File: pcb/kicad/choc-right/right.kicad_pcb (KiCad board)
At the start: 2 copper layers, 135.9 x 90.2 mm, 61 parts, among them J1 USB_C_Receptacle_USB2.0, J2 AudioJack4, J3 Conn_01x12_Male, SW1 BOOT, SW10 SW_Push, SW12 SW_Push, SW13 SW_Push, SW14 SW_Push, SW15 SW_Push, SW17 SW_Push, SW18 SW_Push, SW19 SW_Push, SW2 RESET, SW21 SW_Push, SW22 SW_Push, SW23 SW_Push, SW24 SW_Push, SW3 SW_Push, SW31 SW_Push, SW32 SW_Push, SW33 SW_Push, SW34 SW_Push, SW4 SW_Push, SW5 SW_Push, SW7 SW_Push, SW8 SW_Push, SW9 SW_Push, U1 STM32, U2 LDO

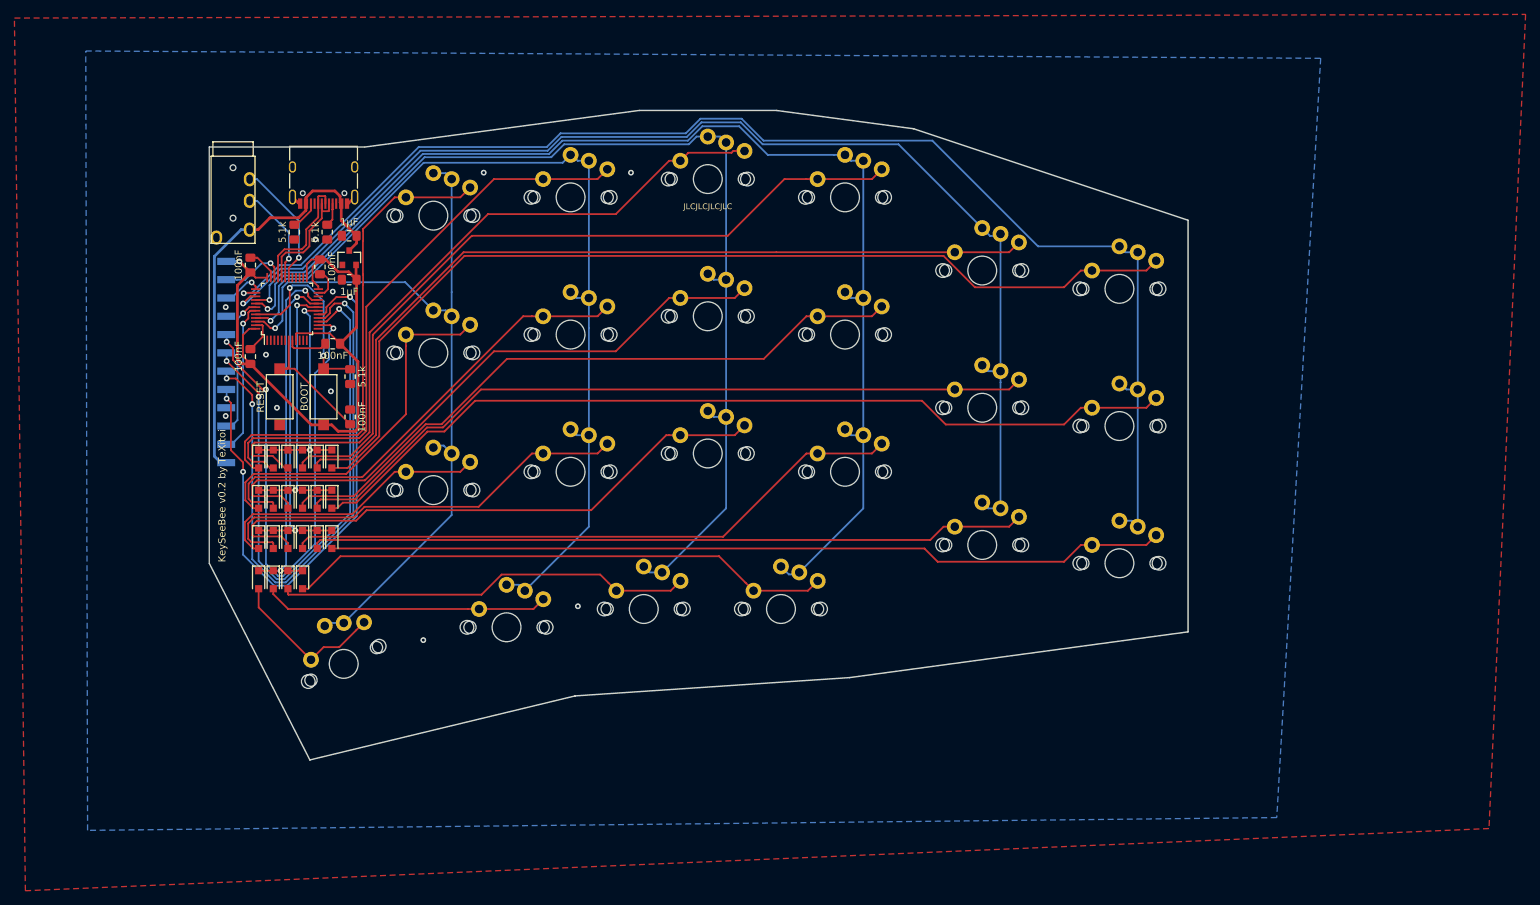
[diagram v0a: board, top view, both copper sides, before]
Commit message: right side.
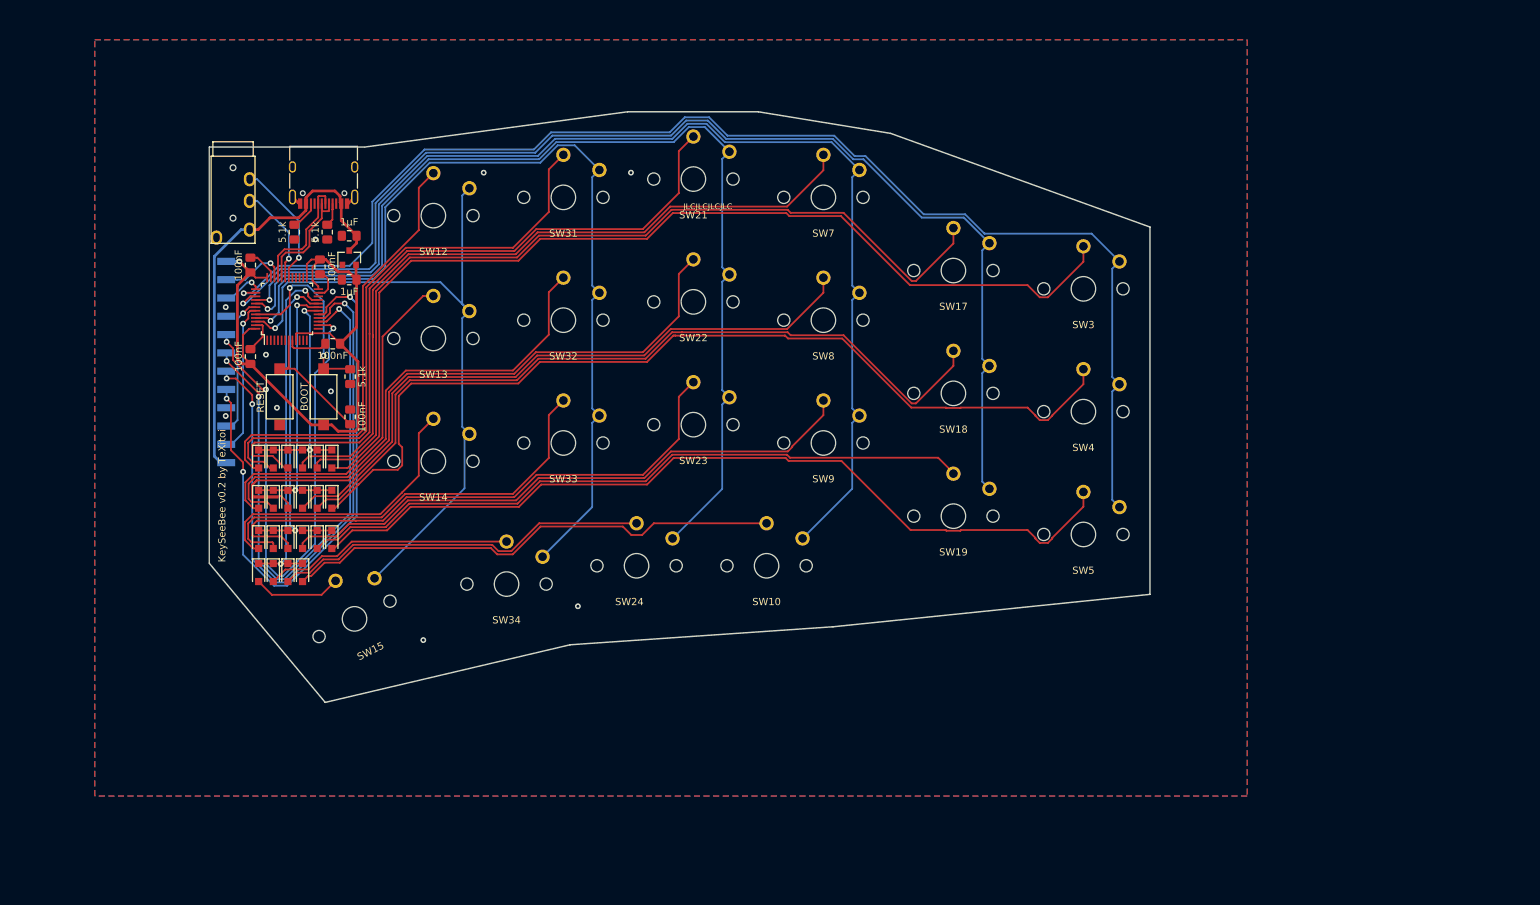
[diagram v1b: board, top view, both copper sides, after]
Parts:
- SW10, SW12, SW13, SW14, SW15, SW17, SW18, SW19, SW21, SW22, SW23, SW24, SW3, SW31, SW32, SW33, SW34, SW4, SW5, SW7, SW8, SW9: footprint custom:CherryMX_Choc_1u -> custom:choc-1
- moved SW15 6.43 mm to (101.1, 130.4)
- moved SW5 6.40 mm to (202.3, 118.7)
- moved SW10 6.32 mm to (158.3, 123.0)
- moved SW24 6.08 mm to (140.2, 123.0)
- moved SW34 6.00 mm to (122.2, 125.6)
- moved SW19 5.66 mm to (184.2, 116.1)
- moved SW4 5.39 mm to (202.3, 101.6)
- moved SW3 5.00 mm to (202.3, 84.6)
- moved SW9 5.00 mm to (166.2, 106.0)
- moved SW18 4.47 mm to (184.2, 99.1)
- moved SW23 4.47 mm to (148.1, 103.4)
- moved SW33 4.12 mm to (130.1, 106.0)
- moved SW14 4.00 mm to (112.0, 108.5)
- moved SW17 4.00 mm to (184.2, 82.0)
- moved SW8 3.61 mm to (166.2, 88.9)
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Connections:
- J1 pad A8: Net-(J1-PadA8) -> (no net)
- J1 pad B8: Net-(J1-PadB8) -> (no net)
- U1 pad 1: VBAT -> (no net)
- U1 pad 10: Net-(U1-Pad10) -> (no net)
- U1 pad 11: Net-(U1-Pad11) -> (no net)
- U1 pad 12: Net-(U1-Pad12) -> (no net)
- U1 pad 13: Net-(U1-Pad13) -> (no net)
- U1 pad 2: Net-(U1-Pad2) -> (no net)
- U1 pad 22: Net-(U1-Pad22) -> (no net)
- U1 pad 26: Net-(U1-Pad26) -> (no net)
- U1 pad 27: Net-(U1-Pad27) -> (no net)
- U1 pad 28: Net-(U1-Pad28) -> (no net)
- U1 pad 29: Net-(U1-Pad29) -> (no net)
- U1 pad 3: Net-(U1-Pad3) -> (no net)
- U1 pad 4: Net-(U1-Pad4) -> (no net)
- U1 pad 5: Net-(U1-Pad5) -> (no net)
- U1 pad 6: Net-(U1-Pad6) -> (no net)
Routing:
- net COL6: track 111.5 -> 98.3 mm
- net Net-(D17-Pad2): track 22.4 -> 12.2 mm
- net COL3: track 167.2 -> 158.7 mm
- net Net-(D24-Pad2): track 87.2 -> 95.5 mm
- net COL1: track 187.5 -> 180.9 mm
- net Net-(D12-Pad2): track 75.9 -> 69.5 mm
- net COL4: track 149.6 -> 143.2 mm
- net Net-(D6-Pad2): track 123.5 -> 129.8 mm
- net Net-(D20-Pad2): track 105.3 -> 110.8 mm
- net Net-(D14-Pad2): track 67.1 -> 61.6 mm
- net Net-(D26-Pad2): track 57.9 -> 52.5 mm
- net COL5: track 131.1 -> 125.7 mm
- net Net-(D19-Pad2): track 118.6 -> 123.7 mm
- net Net-(D36-Pad2): track 39.7 -> 34.7 mm
- net Net-(D21-Pad2): track 99.7 -> 94.8 mm
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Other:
- board size 135.9 x 90.2 mm -> 130.6 x 82 mm
